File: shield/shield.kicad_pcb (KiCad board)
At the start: 2 copper layers, 21.8 x 69.4 mm, 3 parts

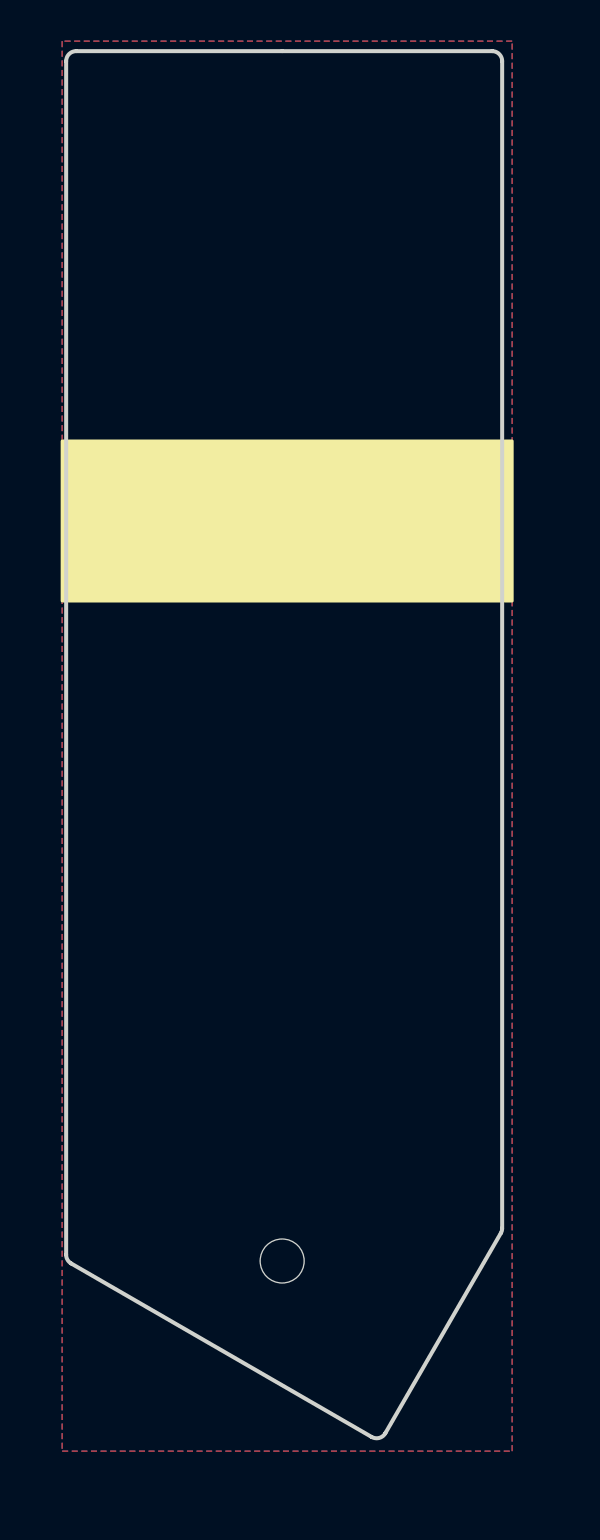
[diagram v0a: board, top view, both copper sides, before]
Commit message: new rev
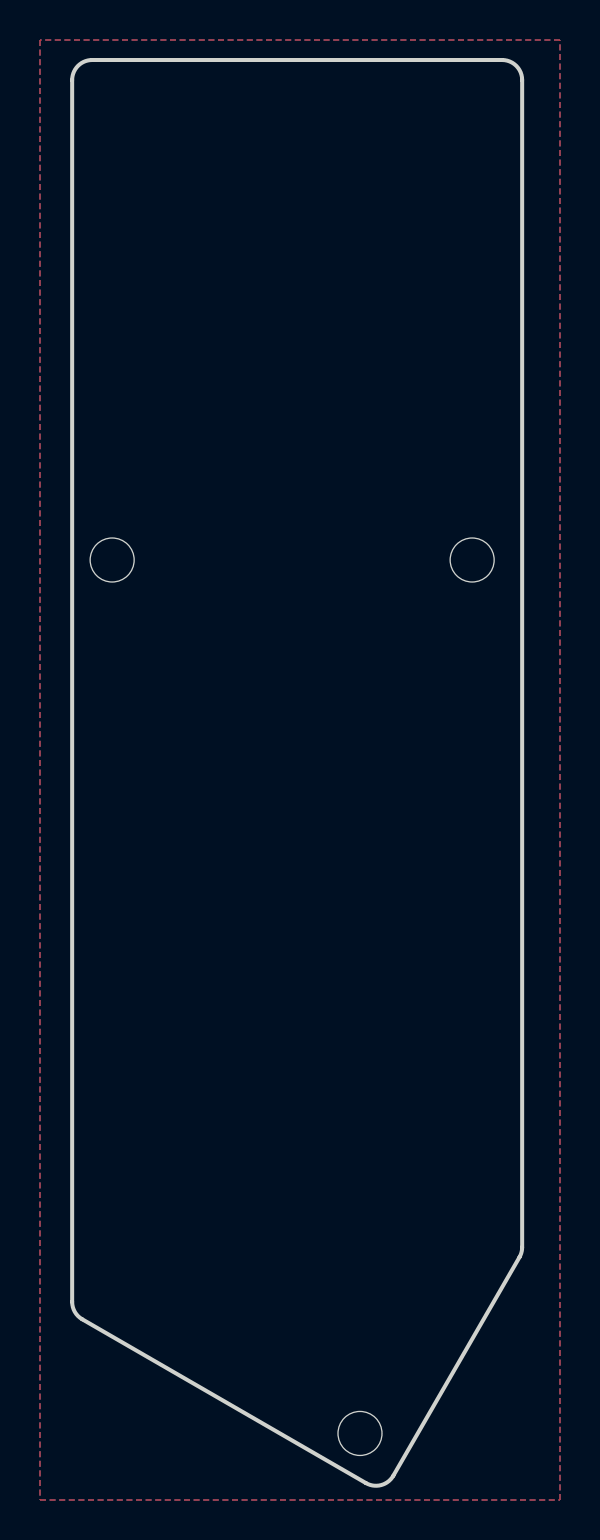
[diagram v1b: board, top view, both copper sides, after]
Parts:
- H1, H2, H3: footprint s1:Hole_2.2mm -> one:Hole_2.2mm
- moved H1 47.3 mm to (203.9, 135.9)
- moved H3 36.1 mm to (191.5, 92.3)
- moved H2 2.19 mm to (209.5, 92.3)
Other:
- board size 21.8 x 69.4 mm -> 22.5 x 71.3 mm
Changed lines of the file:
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@@
     )
     (pad_to_mask_clearance 0)
-    (aux_axis_origin 191.5 90.303907)
-    (grid_origin 191.5 90.303907)
+    (aux_axis_origin 191.5 92.253468)
+    (grid_origin 203.89201 135.926214)
     (pcbplotparams
       (layerselection 0x00010fc_ffffffff)
@@
   )
   (net 0 "")
-  (footprint "s1:Hole_2.2mm" (layer "F.Cu")
-    (at 208.5 90.303907)
+  (footprint "one:Hole_2.2mm" (layer "F.Cu")
+    (at 191.5 92.253468)
+    (property "Sheetfile" "shield.kicad_sch")
+    (property "Sheetname" "")
+    (property "ki_description" "Mounting Hole without connection")
+    (property "ki_keywords" "mounting hole")
+    (attr through_hole)
+    (fp_text reference "H3" (at 0 0) (layer "F.Fab") hide
+        (effects (font (size 1 1) (thickness 0.15)))
+    )
+    (fp_text value "StandoffHole" (at 0 0) (layer "F.Fab") hide
+        (effects (font (size 1 1) (thickness 0.15)))
+    )
+    (fp_circle (center 0 0) (end 0 -1.6)
+      (stroke (width 0.12) (type solid)) (fill none) (layer "B.CrtYd"))
+    (fp_circle (center 0 0) (end 0 -1.6)
+      (stroke (width 0.12) (type solid)) (fill none) (layer "F.CrtYd"))
+    (pad "" np_thru_hole circle (at 0 0 270) (size 2.2 2.2) (drill 2.2) (layers "F&B.Cu" "*.Mask"))
+  )
+  (footprint "one:Hole_2.2mm" (layer "F.Cu")
+    (at 203.89201 135.926214)
+    (property "Sheetfile" "shield.kicad_sch")
+    (property "Sheetname" "")
+    (property "ki_description" "Mounting Hole without connection")
+    (property "ki_keywords" "mounting hole")
+    (attr through_hole)
+    (fp_text reference "H1" (at 0 0) (layer "F.Fab") hide
+        (effects (font (size 1 1) (thickness 0.15)))
+    )
+    (fp_text value "StandoffHole" (at 0 0) (layer "F.Fab") hide
+        (effects (font (size 1 1) (thickness 0.15)))
+    )
+    (fp_circle (center 0 0) (end 0 -1.6)
+      (stroke (width 0.12) (type solid)) (fill none) (layer "B.CrtYd"))
+    (fp_circle (center 0 0) (end 0 -1.6)
+      (stroke (width 0.12) (type solid)) (fill none) (layer "F.CrtYd"))
+    (pad "" np_thru_hole circle (at 0 0 270) (size 2.2 2.2) (drill 2.2) (layers "F&B.Cu" "*.Mask"))
+  )
+  (footprint "one:Hole_2.2mm" (layer "F.Cu")
+    (at 209.5 92.253468)
     (property "Sheetfile" "shield.kicad_sch")
     (property "Sheetname" "")
@@
     (fp_circle (center 0 0) (end 0 -1.6)
       (stroke (width 0.12) (type solid)) (fill none) (layer "F.CrtYd"))
-    (pad "" np_thru_hole circle (at 0 0 270) (size 2.2 2.2) (drill 2.2) (layers "*.Cu" "*.Mask"))
+    (pad "" np_thru_hole circle (at 0 0 270) (size 2.2 2.2) (drill 2.2) (layers "F&B.Cu" "*.Mask"))
   )
-  (footprint "s1:Hole_2.2mm" (layer "F.Cu")
-    (at 191.5 90.303907)
-    (property "Sheetfile" "shield.kicad_sch")
-    (property "Sheetname" "")
-    (property "ki_description" "Mounting Hole without connection")
-    (property "ki_keywords" "mounting hole")
-    (attr through_hole)
-    (fp_text reference "H1" (at 0 0) (layer "F.Fab") hide
-        (effects (font (size 1 1) (thickness 0.15)))
-    )
-    (fp_text value "StandoffHole" (at 0 0) (layer "F.Fab") hide
-        (effects (font (size 1 1) (thickness 0.15)))
-    )
-    (fp_circle (center 0 0) (end 0 -1.6)
-      (stroke (width 0.12) (type solid)) (fill none) (layer "B.CrtYd"))
-    (fp_circle (center 0 0) (end 0 -1.6)
-      (stroke (width 0.12) (type solid)) (fill none) (layer "F.CrtYd"))
-    (pad "" np_thru_hole circle (at 0 0 270) (size 2.2 2.2) (drill 2.2) (layers "*.Cu" "*.Mask"))
-  )
-  (footprint "s1:Hole_2.2mm" (layer "F.Cu")
-    (at 199.999999 127.303907)
-    (property "Sheetfile" "shield.kicad_sch")
-    (property "Sheetname" "")
-    (property "ki_description" "Mounting Hole without connection")
-    (property "ki_keywords" "mounting hole")
-    (attr through_hole)
-    (fp_text reference "H3" (at 0 0) (layer "F.Fab") hide
-        (effects (font (size 1 1) (thickness 0.15)))
-    )
-    (fp_text value "StandoffHole" (at 0 0) (layer "F.Fab") hide
-        (effects (font (size 1 1) (thickness 0.15)))
-    )
-    (fp_circle (center 0 0) (end 0 -1.6)
-      (stroke (width 0.12) (type solid)) (fill none) (layer "B.CrtYd"))
-    (fp_circle (center 0 0) (end 0 -1.6)
-      (stroke (width 0.12) (type solid)) (fill none) (layer "F.CrtYd"))
-    (pad "" np_thru_hole circle (at 0 0 270) (size 2.2 2.2) (drill 2.2) (layers "*.Cu" "*.Mask"))
-  )
-  (gr_poly
-    (pts
-      (xy 211.5 86.303907)
-      (xy 189 86.303907)
-      (xy 189 94.303907)
-      (xy 211.5 94.303907)
-    )
-    (stroke (width 0.15) (type solid)) (fill solid) (layer "B.SilkS"))
-  (gr_poly
-    (pts
-      (xy 189 86.303907)
-      (xy 211.5 86.303907)
-      (xy 211.5 94.303907)
-      (xy 189 94.303907)
-    )
-    (stroke (width 0.15) (type solid)) (fill solid) (layer "F.SilkS"))
-  (gr_circle (center 191.5 90.303907) (end 192.5 90.303907)
-    (stroke (width 0.2) (type solid)) (fill none) (layer "Eco2.User"))
-  (gr_circle (center 199.999999 127.303907) (end 200.999999 127.303907)
-    (stroke (width 0.2) (type solid)) (fill none) (layer "Eco2.User"))
-  (gr_circle (center 208.5 90.303907) (end 209.5 90.303907)
-    (stroke (width 0.2) (type solid)) (fill none) (layer "Eco2.User"))
-  (gr_arc (start 189.2 67.310734) (mid 189.346444 66.957175) (end 189.7 66.810734)
+  (gr_line (start 211 67.253468) (end 190.5 67.253468)
     (stroke (width 0.2) (type solid)) (layer "Edge.Cuts"))
-  (gr_arc (start 211 125.663105) (mid 210.982968 125.792517) (end 210.933013 125.913105)
+  (gr_line (start 205.557073 138.042239) (end 211.866025 127.114814)
     (stroke (width 0.2) (type solid)) (layer "Edge.Cuts"))
-  (gr_arc (start 205.157073 135.917326) (mid 204.853475 136.150263) (end 204.474061 136.100338)
+  (gr_line (start 212 126.614814) (end 212 68.253468)
     (stroke (width 0.2) (type solid)) (layer "Edge.Cuts"))
-  (gr_line (start 189.7 66.810734) (end 200 66.810734)
+  (gr_arc (start 189.5 68.253468) (mid 189.79289 67.546356) (end 190.5 67.253468)
     (stroke (width 0.2) (type solid)) (layer "Edge.Cuts"))
-  (gr_line (start 204.474061 136.100338) (end 189.45 127.426193)
+  (gr_arc (start 212 126.614814) (mid 211.965937 126.873638) (end 211.866025 127.114814)
     (stroke (width 0.2) (type solid)) (layer "Edge.Cuts"))
-  (gr_line (start 189.2 126.99318) (end 189.2 67.310734)
+  (gr_arc (start 190 130.215059) (mid 189.633985 129.849032) (end 189.5 129.349034)
     (stroke (width 0.2) (type solid)) (layer "Edge.Cuts"))
-  (gr_arc (start 210.5 66.810734) (mid 210.853551 66.957181) (end 211 67.310734)
+  (gr_line (start 190 130.215059) (end 204.191048 138.408265)
     (stroke (width 0.2) (type solid)) (layer "Edge.Cuts"))
-  (gr_line (start 200 66.810734) (end 210.5 66.810734)
+  (gr_arc (start 205.557073 138.042239) (mid 204.949862 138.508206) (end 204.191048 138.408265)
     (stroke (width 0.2) (type solid)) (layer "Edge.Cuts"))
-  (gr_line (start 211 67.310734) (end 211 125.663105)
+  (gr_arc (start 211 67.253468) (mid 211.707104 67.546362) (end 212 68.253468)
     (stroke (width 0.2) (type solid)) (layer "Edge.Cuts"))
-  (gr_arc (start 189.45 127.426193) (mid 189.267004 127.243176) (end 189.2 126.99318)
+  (gr_line (start 189.5 68.253468) (end 189.5 129.349034)
     (stroke (width 0.2) (type solid)) (layer "Edge.Cuts"))
-  (gr_line (start 210.933013 125.913105) (end 205.157073 135.917326)
-    (stroke (width 0.2) (type solid)) (layer "Edge.Cuts"))
+  (gr_circle (center 191.5 92.253468) (end 192.5 92.253468)
+    (stroke (width 0.2) (type solid)) (fill none) (layer "User.9"))
+  (gr_circle (center 203.89201 135.926214) (end 204.89201 135.926214)
+    (stroke (width 0.2) (type solid)) (fill none) (layer "User.9"))
+  (gr_circle (center 209.5 92.253468) (end 210.5 92.253468)
+    (stroke (width 0.2) (type solid)) (fill none) (layer "User.9"))
   (zone (net 0) (net_name "") (layers "F&B.Cu") (hatch edge 0.5)
     (connect_pads (clearance 0.2))
@@
     (polygon
       (pts
-        (xy 211.5 66.310734)
-        (xy 189 66.310734)
-        (xy 189 136.810734)
-        (xy 211.5 136.810734)
+        (xy 213.89201 66.253468)
+        (xy 187.89201 66.253468)
+        (xy 187.89201 139.253468)
+        (xy 213.89201 139.253468)
       )
     )
-  )
-  (zone (net 0) (net_name "") (layers "F&B.Cu") (hatch edge 0.5)
-    (connect_pads (clearance 0))
-    (min_thickness 0.25) (filled_areas_thickness no)
-    (keepout (tracks allowed) (vias allowed) (pads allowed) (copperpour not_allowed) (footprints allowed))
-    (fill (thermal_gap 0.5) (thermal_bridge_width 0.5))
-    (polygon
-      (pts
-        (xy 189 86.310734)
-        (xy 211.5 86.310734)
-        (xy 211.5 94.310734)
-        (xy 189 94.310734)
-      )
-    )
